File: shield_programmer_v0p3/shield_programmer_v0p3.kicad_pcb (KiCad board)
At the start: 2 copper layers, 72.4 x 53.3 mm, 3 parts, among them P1 CONN_3X2

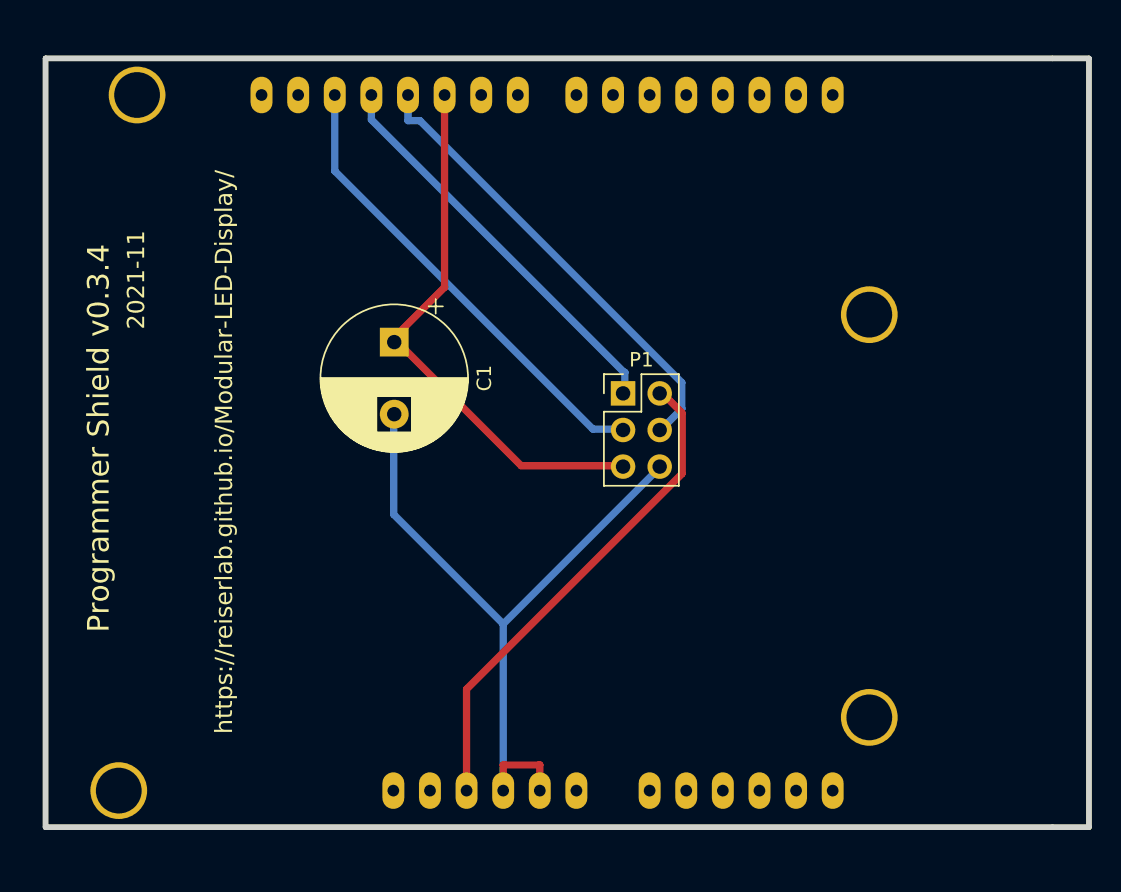
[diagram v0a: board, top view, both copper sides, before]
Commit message: update shield_programmer
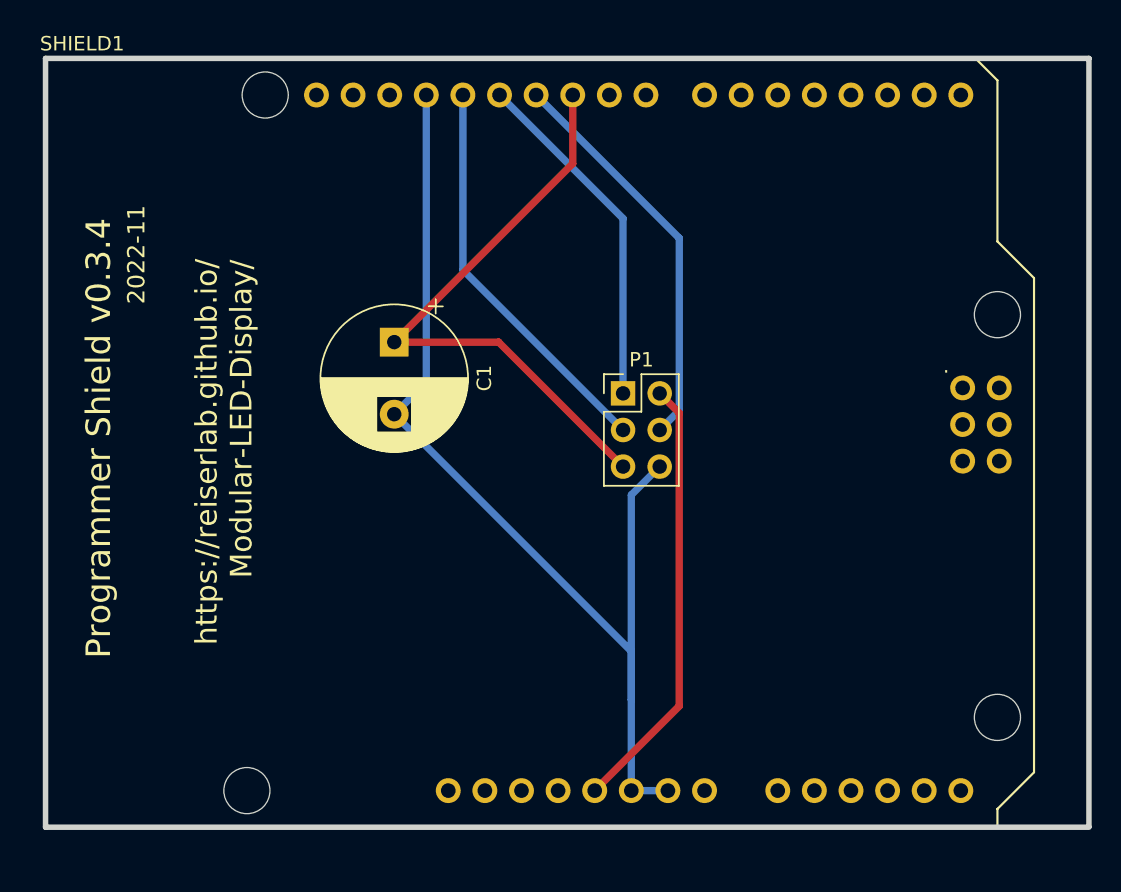
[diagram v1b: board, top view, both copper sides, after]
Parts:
- C1: value CP1 -> 10uF
- SHIELD1: footprint shield_programmer_v0p3:ARDUINO_SHIELD -> Arduino:Arduino_Zero_Shield
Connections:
- C1 pad 2: /GND -> GND
- P1 pad 2: /5V -> +5V
- P1 pad 6: /GND -> GND
- SHIELD1 pad 3V3: (no net) -> unconnected-(SHIELD1-Pad3V3)
- SHIELD1 pad AREF: (no net) -> unconnected-(SHIELD1-PadAREF)
- SHIELD1 pad GND1: /GND -> GND
- SHIELD1 pad GND2: /GND -> GND
- SHIELD1 pad GND3: (no net) -> GND
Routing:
- net GND: track 0.00 -> 75.5 mm
- net /GND: track 51.1 -> 0.00 mm
- net /5V: track 34.4 -> 0.00 mm
- net +5V: track 0.00 -> 30.6 mm
- net /SCK: track 32.8 -> 27.8 mm
- net /COPI: track 32.1 -> 27.9 mm
- net /RST: track 37.9 -> 42.0 mm
- net /CIPO: track 28.0 -> 24.3 mm
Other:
- net class Default removed
- board text added: "2022-11"
- board text added: "https://reiserlab.github.io/ Modular-LED-Display/"
- board text removed: "2021-11"
- board text removed: "https://reiserlab.github.io/Modular-LED-Display/"
